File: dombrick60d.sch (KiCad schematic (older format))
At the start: 147 parts, among them J1 AVR-ISP-6, SW1 SW_Push, U1 ATmega32U2-AU, U2 PRTR5V0U2X, Y1 16MHz

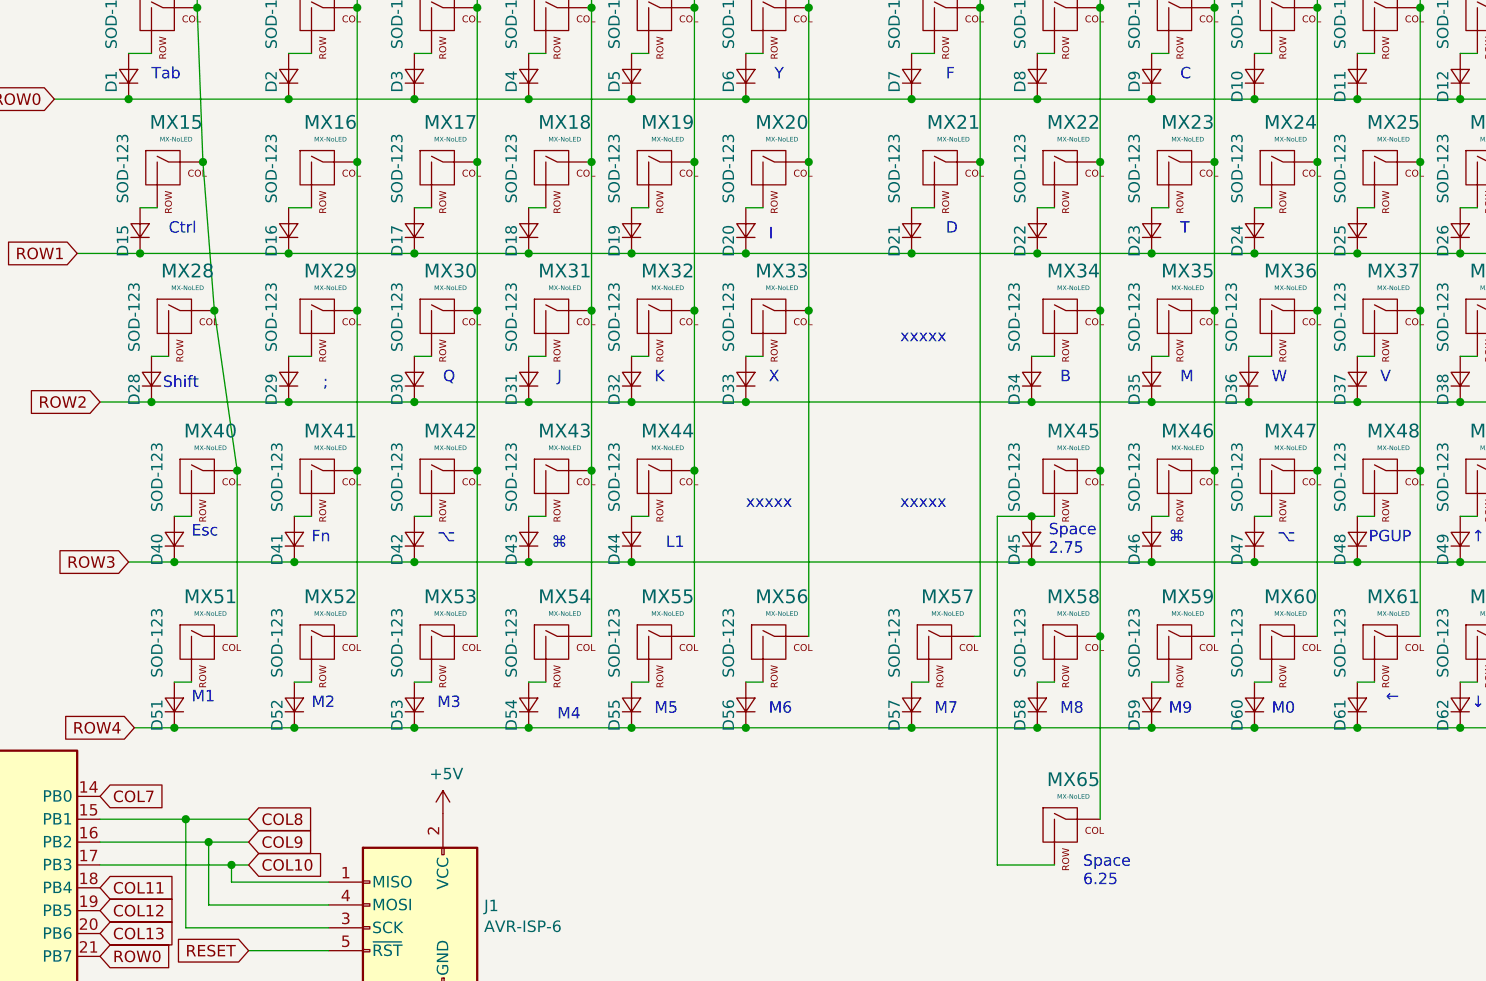
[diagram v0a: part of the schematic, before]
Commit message: sugee ganbatta
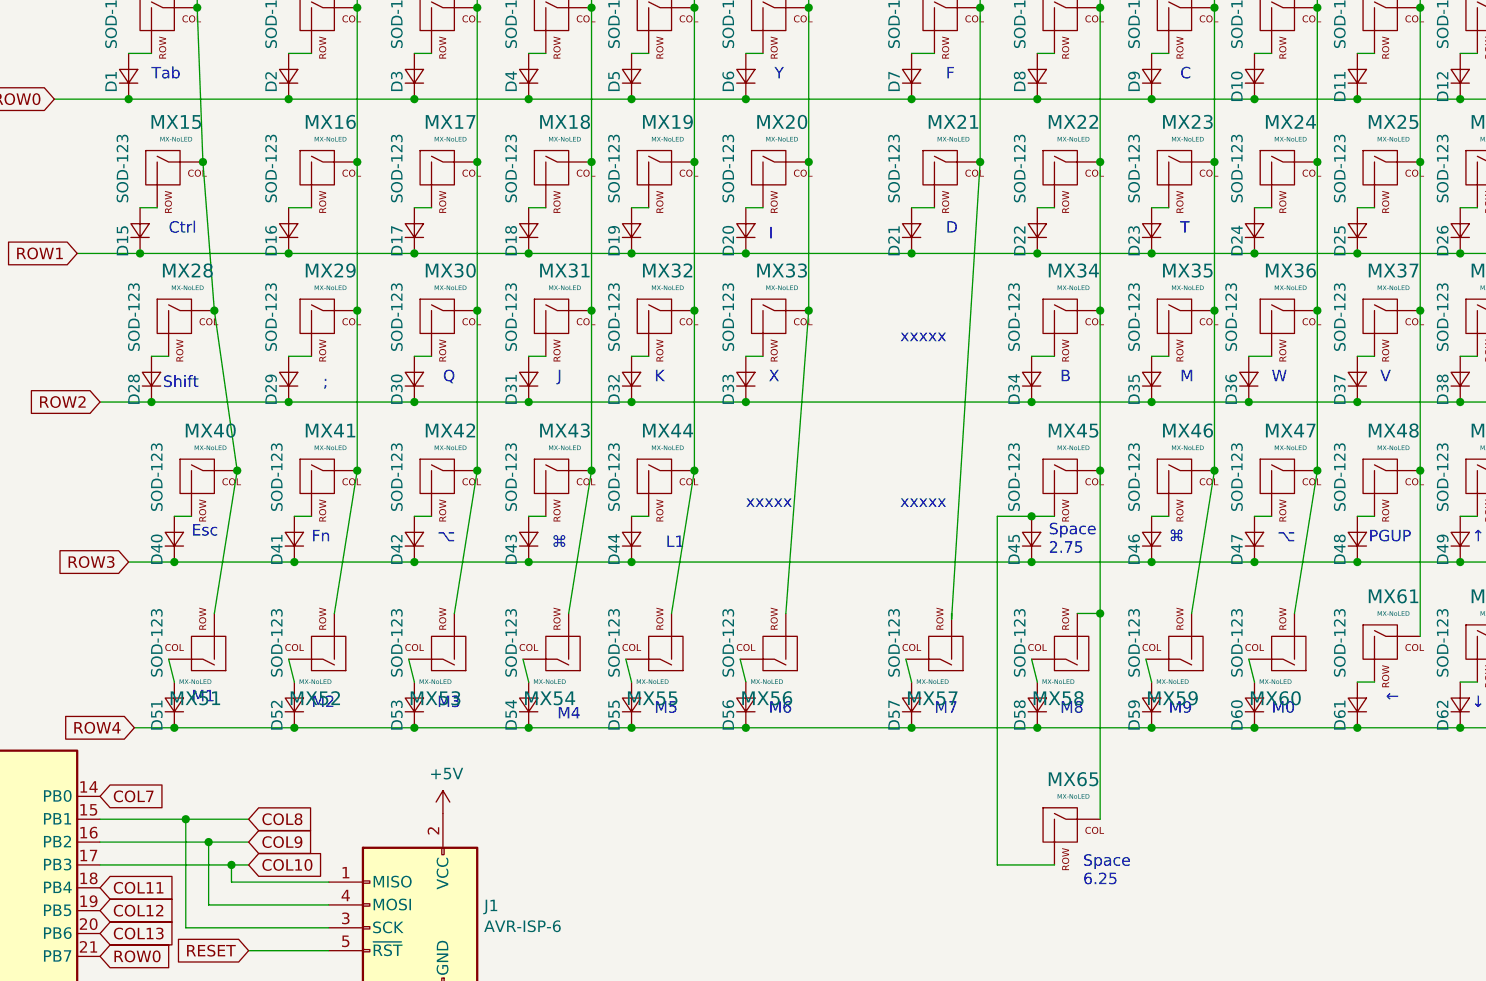
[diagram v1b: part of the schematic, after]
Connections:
- net COL0: now also MX51.2 (ROW); no longer MX51.1 (COL)
- net COL1: now also MX52.2 (ROW); no longer MX52.1 (COL)
- net COL2: now also MX53.2 (ROW); no longer MX53.1 (COL)
- net COL3: now also MX54.2 (ROW); no longer MX54.1 (COL)
- net COL4: now also MX55.2 (ROW); no longer MX55.1 (COL)
- net COL5: now also MX56.2 (ROW); no longer MX56.1 (COL)
- net COL6: now also MX57.2 (ROW); no longer MX57.1 (COL)
- net COL7: now also MX58.2 (ROW); no longer MX58.1 (COL)
- net COL8: now also MX59.2 (ROW); no longer MX59.1 (COL)
- net COL9: now also MX60.2 (ROW); no longer MX60.1 (COL)
- net at D55.2 (A): now also MX55.1 (COL); no longer MX55.2 (ROW)
- net at D59.2 (A): now also MX59.1 (COL); no longer MX59.2 (ROW)
- net at D60.2 (A): now also MX60.1 (COL); no longer MX60.2 (ROW)
- net at D51.2 (A): now also MX51.1 (COL); no longer MX51.2 (ROW)
- net at D52.2 (A): now also MX52.1 (COL); no longer MX52.2 (ROW)
- net at D53.2 (A): now also MX53.1 (COL); no longer MX53.2 (ROW)
- net at D54.2 (A): now also MX54.1 (COL); no longer MX54.2 (ROW)
- net at D56.2 (A): now also MX56.1 (COL); no longer MX56.2 (ROW)
- net at D57.2 (A): now also MX57.1 (COL); no longer MX57.2 (ROW)
- net at D58.2 (A): now also MX58.1 (COL); no longer MX58.2 (ROW)
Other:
- moved on the sheet: MX51, MX52, MX53, MX54, MX55, MX56, MX57, MX58, MX59, MX60
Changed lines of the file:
@@
 	9300 3600 9750 3600
 Wire Wire Line
-	8675 3200 8675 3925
+	8675 3200 8575 3825
 Wire Wire Line
 	8400 3400 8475 3400
@@
 Data
 89 50 4E 47 0D 0A 1A 0A 00 00 00 0D 49 48 44 52 00 00 01 AC 00 00 00 BB 08 02 00 00 00 B6 0E 3D
-6C 00 00 00 03 73 42 49 54 08 08 08 DB E1 4F E0 00 00 00 09 70 48 59 73 00 00 0B 12 00 00 0B 12
-01 D2 DD 7E FC 00 00 20 00 49 44 41 54 78 9C ED 9D 3F 7C 1A C9 15 C7 67 51 CA 58 0B E9 4F 80 7B
+6C 00 00 00 03 73 42 49 54 08 08 08 DB E1 4F E0 00 00 00 09 70 48 59 73 00 00 0A F0 00 00 0A F0
+01 42 AC 34 98 00 00 20 00 49 44 41 54 78 9C ED 9D 3F 7C 1A C9 15 C7 67 51 CA 58 0B E9 4F 80 7B
 F3 C7 9F B4 16 8B D2 0B AC 4B 1B 49 F8 EA 33 C8 57 5B 20 5F 9B 48 C8 A9 83 B0 9D 2E 9F 08 64 7F
 52 5A AC E4 94 39 81 7C 2E 73 06 E4 DE FC 71 CA 13 93 E2 99 F1 63 76 C1 48 62 97 85 7D DF 42 9F
@@
 F 3 "" H 5625 3950 60  0001 C CNN
 	1    6250 3975
-	1    0    0    -1
+	-1   0    0    1
 $EndComp
 $Comp
@@
 $EndComp
 Wire Wire Line
-	6125 4125 6200 4125
+	6125 4125 6100 4025
 Text Notes 6225 4275 0    50   ~ 0
 M5
@@
 $EndComp
 $Comp
-L MX_Alps_Hybrid:MX-NoLED MX?
-U 1 1 5E9D839C
-P 9425 3975
-AR Path="/5E22FDCD/5E9D839C" Ref="MX?"  Part="1"
-AR Path="/5E9D839C" Ref="MX61"  Part="1"
-F 0 "MX61" H 9458 4198 60  0000 C CNN
-F 1 "MX-NoLED" H 9458 4124 20  0000 C CNN
-F 2 "MX_Alps_Hybrid:MX-1U-NoLED" H 8800 3950 60  0001 C CNN
-F 3 "" H 8800 3950 60  0001 C CNN
-	1    9425 3975
-	1    0    0    -1
-$EndComp
-$Comp
 L Device:D_Small D?
 U 1 1 5E9D83A6
@@
 →
 Wire Wire Line
-	8850 4125 8925 4125
+	8850 4125 8825 4025
 $Comp
 L MX_Alps_Hybrid:MX-NoLED MX?
@@
 F 3 "" H 8350 3950 60  0001 C CNN
 	1    8975 3975
-	1    0    0    -1
+	-1   0    0    1
 $EndComp
 $Comp
@@
 F 3 "" H 7900 3950 60  0001 C CNN
 	1    8525 3975
-	1    0    0    -1
-$EndComp
-Wire Wire Line
-	8400 4125 8475 4125
+	-1   0    0    1
+$EndComp
+Wire Wire Line
+	8400 4125 8375 4025
 Text Notes 5800 4300 0    50   ~ 0
 M4
@@
 F 3 "" H 3625 3950 60  0001 C CNN
 	1    4250 3975
-	1    0    0    -1
+	-1   0    0    1
 $EndComp
 $Comp
@@
 $EndComp
 Wire Wire Line
-	4125 4125 4200 4125
+	4125 4125 4100 4025
 $Comp
 L MX_Alps_Hybrid:MX-NoLED MX?
@@
 F 3 "" H 4150 3950 60  0001 C CNN
 	1    4775 3975
-	1    0    0    -1
+	-1   0    0    1
 $EndComp
 $Comp
@@
 $EndComp
 Wire Wire Line
-	4650 4125 4725 4125
+	4650 4125 4625 4025
 $Comp
 L MX_Alps_Hybrid:MX-NoLED MX?
@@
 F 3 "" H 4675 3950 60  0001 C CNN
 	1    5300 3975
-	1    0    0    -1
+	-1   0    0    1
 $EndComp
 $Comp
@@
 $EndComp
 Wire Wire Line
-	5175 4125 5250 4125
+	5175 4125 5150 4025
 $Comp
 L MX_Alps_Hybrid:MX-NoLED MX?
@@
 F 3 "" H 5175 3950 60  0001 C CNN
 	1    5800 3975
-	1    0    0    -1
+	-1   0    0    1
 $EndComp
 $Comp
@@
 $EndComp
 Wire Wire Line
-	5675 4125 5750 4125
+	5675 4125 5650 4025
 Text Notes 4200 4225 0    50   ~ 0
 M1
@@
 F 3 "" H 6125 3950 60  0001 C CNN
 	1    6750 3975
-	1    0    0    -1
+	-1   0    0    1
 $EndComp
 $Comp
@@
 $EndComp
 Wire Wire Line
-	6625 4125 6700 4125
+	6625 4125 6600 4025
 Text Notes 6725 4275 0    50   ~ 0
 M6
@@
 F 3 "" H 6850 3950 60  0001 C CNN
 	1    7475 3975
-	1    0    0    -1
+	-1   0    0    1
 $EndComp
 $Comp
@@
 $EndComp
 Wire Wire Line
-	7350 4125 7425 4125
+	7350 4125 7325 4025
 Text Notes 7450 4275 0    50   ~ 0
 M7
@@
 F 3 "" H 7400 3950 60  0001 C CNN
 	1    8025 3975
-	1    0    0    -1
+	-1   0    0    1
 $EndComp
 $Comp
@@
 $EndComp
 Wire Wire Line
-	7900 4125 7975 4125
+	7900 4125 7875 4025
 Text Notes 8000 4275 0    50   ~ 0
 M8
@@
 	7900 4325 8400 4325
 Wire Wire Line
-	4400 3200 4400 3925
+	4400 3200 4300 3825
 Connection ~ 4400 3200
 Wire Wire Line
-	4925 3200 4925 3925
+	4925 3200 4825 3825
 Connection ~ 4925 3200
 Wire Wire Line
-	5450 3200 5450 3925
+	5450 3200 5350 3825
 Connection ~ 5450 3200
 Wire Wire Line
-	6900 3925 6900 2500
+	6800 3825 6900 2500
 Connection ~ 6900 2500
 Wire Wire Line
@@
 	11025 800  11025 1175
 Wire Wire Line
-	8175 3200 8175 3925
-Connection ~ 8175 3925
-Wire Wire Line
-	8175 3925 8175 4725
-Wire Wire Line
-	7650 3925 7625 3925
-Wire Wire Line
-	5950 3200 5950 3925
+	7525 3850 7525 3825
+Wire Wire Line
+	5950 3200 5850 3825
 Connection ~ 5950 3200
 Wire Wire Line
-	6400 3200 6400 3925
+	6400 3200 6300 3825
 Connection ~ 6400 3200
 Connection ~ 8175 3200
@@
 Connection ~ 7650 1850
 Wire Wire Line
-	7650 1850 7650 3925
+	7650 1850 7525 3850
 Text Notes 7300 2650 0    50   ~ 0
 xxxxx
 Wire Wire Line
-	9125 3200 9125 3925
+	9125 3200 9025 3825
 Connection ~ 9125 3200
 Wire Wire Line
@@
 Text GLabel 2100 4625 0    50   Input ~ 0
 RESET
+Wire Wire Line
+	8175 3200 8175 3825
+Wire Wire Line
+	8075 3825 8175 3825
+Connection ~ 8175 3825
+Wire Wire Line
+	8175 3825 8175 4725
+$Comp
+L MX_Alps_Hybrid:MX-NoLED MX?
+U 1 1 5E9D839C
+P 9425 3975
+AR Path="/5E22FDCD/5E9D839C" Ref="MX?"  Part="1"
+AR Path="/5E9D839C" Ref="MX61"  Part="1"
+F 0 "MX61" H 9458 4198 60  0000 C CNN
+F 1 "MX-NoLED" H 9458 4124 20  0000 C CNN
+F 2 "MX_Alps_Hybrid:MX-1U-NoLED" H 8800 3950 60  0001 C CNN
+F 3 "" H 8800 3950 60  0001 C CNN
+	1    9425 3975
+	1    0    0    -1
+$EndComp
 $EndSCHEMATC

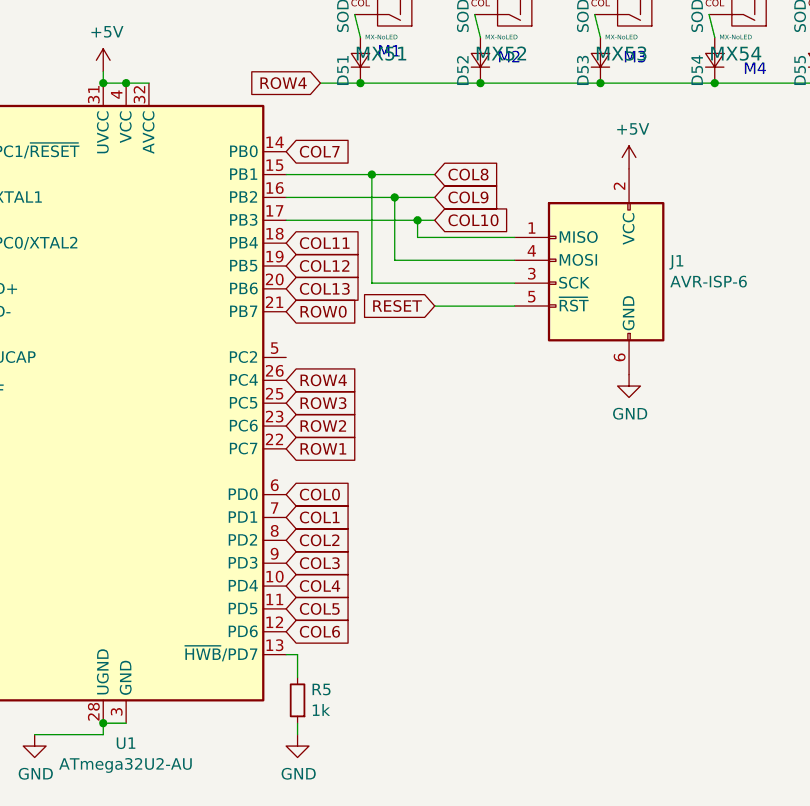
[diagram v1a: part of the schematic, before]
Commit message: sugoku ganbatta
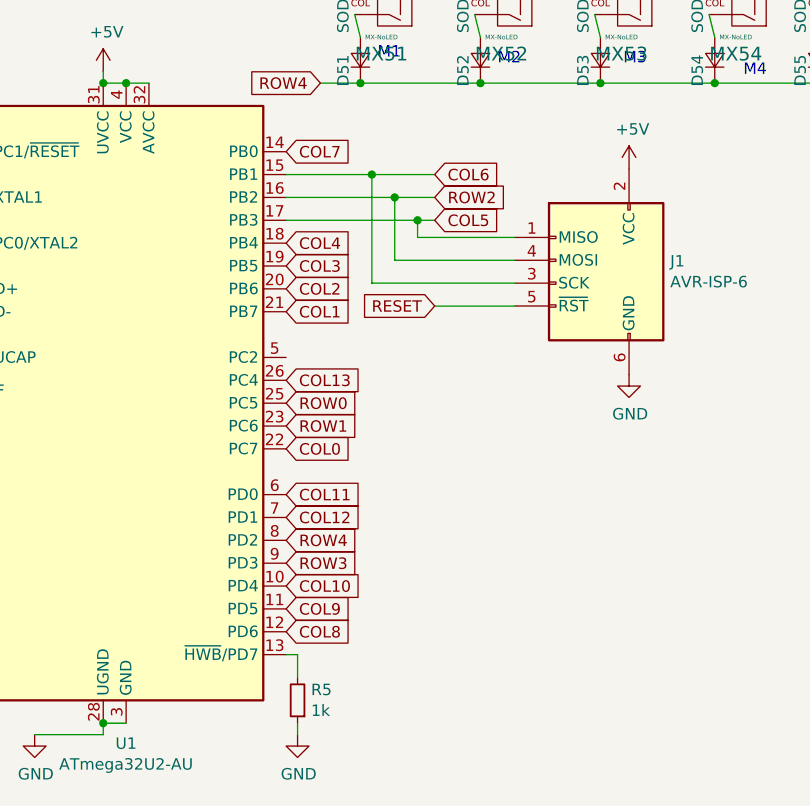
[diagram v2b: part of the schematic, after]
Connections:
- net COL0: now also U1.22 (PC7); no longer U1.6 (PD0)
- net COL1: now also U1.21 (PB7); no longer U1.7 (PD1)
- net COL10: now also U1.10 (PD4); no longer J1.1 (MISO), U1.17 (PB3)
- net COL11: now also U1.6 (PD0); no longer U1.18 (PB4)
- net COL12: now also U1.7 (PD1); no longer U1.19 (PB5)
- net COL13: now also U1.26 (PC4); no longer U1.20 (PB6)
- net COL2: now also U1.20 (PB6); no longer U1.8 (PD2)
- net COL3: now also U1.19 (PB5); no longer U1.9 (PD3)
- net COL4: now also U1.18 (PB4); no longer U1.10 (PD4)
- net COL5: now also J1.1 (MISO), U1.17 (PB3); no longer U1.11 (PD5)
- net COL6: now also J1.3 (SCK), U1.15 (PB1); no longer U1.12 (PD6)
- net COL8: now also U1.12 (PD6); no longer J1.3 (SCK), U1.15 (PB1)
- net COL9: now also U1.11 (PD5); no longer J1.4 (MOSI), U1.16 (PB2)
- net ROW0: now also U1.25 (PC5); no longer U1.21 (PB7)
- net ROW1: now also U1.23 (PC6); no longer U1.22 (PC7)
- net ROW2: now also J1.4 (MOSI), U1.16 (PB2); no longer U1.23 (PC6)
- net ROW3: now also U1.9 (PD3); no longer U1.25 (PC5)
- net ROW4: now also U1.8 (PD2); no longer U1.26 (PC4)
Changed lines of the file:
@@
 EESchema Schematic File Version 4
+LIBS:dombrick60d-cache
 EELAYER 30 0
 EELAYER END
@@
 	4450 5300 4800 5300
 Text GLabel 3800 6125 2    50   Input ~ 0
-COL0
+COL11
 Text GLabel 3800 6225 2    50   Input ~ 0
-COL1
-Text GLabel 3800 6325 2    50   Input ~ 0
-COL2
+COL12
 Text GLabel 3800 6425 2    50   Input ~ 0
-COL3
-Text GLabel 3800 6525 2    50   Input ~ 0
-COL4
-Text GLabel 3800 6625 2    50   Input ~ 0
-COL5
+ROW3
 Text GLabel 3800 6725 2    50   Input ~ 0
-COL6
+COL8
 Text GLabel 3800 4625 2    50   Input ~ 0
 COL7
 Text GLabel 4450 4725 2    50   Input ~ 0
-COL8
+COL6
 Text GLabel 4450 4825 2    50   Input ~ 0
-COL9
+ROW2
 Text GLabel 4450 4925 2    50   Input ~ 0
-COL10
+COL5
 Wire Wire Line
 	4450 4725 4175 4725
@@
 Connection ~ 4375 4925
 Text GLabel 3800 5025 2    50   Input ~ 0
-COL11
+COL4
 Text GLabel 3800 5125 2    50   Input ~ 0
-COL12
+COL3
 Text GLabel 3800 5225 2    50   Input ~ 0
-COL13
-Text GLabel 3800 5325 2    50   Input ~ 0
-ROW0
-Text GLabel 3800 5925 2    50   Input ~ 0
-ROW1
+COL2
 Text GLabel 3800 5825 2    50   Input ~ 0
-ROW2
+ROW1
 Text GLabel 3800 5725 2    50   Input ~ 0
-ROW3
+ROW0
 Text GLabel 3800 5625 2    50   Input ~ 0
-ROW4
+COL13
 Text GLabel 2100 4625 0    50   Input ~ 0
 RESET
@@
 	1    0    0    -1
 $EndComp
+Text GLabel 3800 6325 2    50   Input ~ 0
+ROW4
+Text GLabel 3800 5325 2    50   Input ~ 0
+COL1
+Text GLabel 3800 5925 2    50   Input ~ 0
+COL0
+Text GLabel 3800 6525 2    50   Input ~ 0
+COL10
+Text GLabel 3800 6625 2    50   Input ~ 0
+COL9
 $EndSCHEMATC

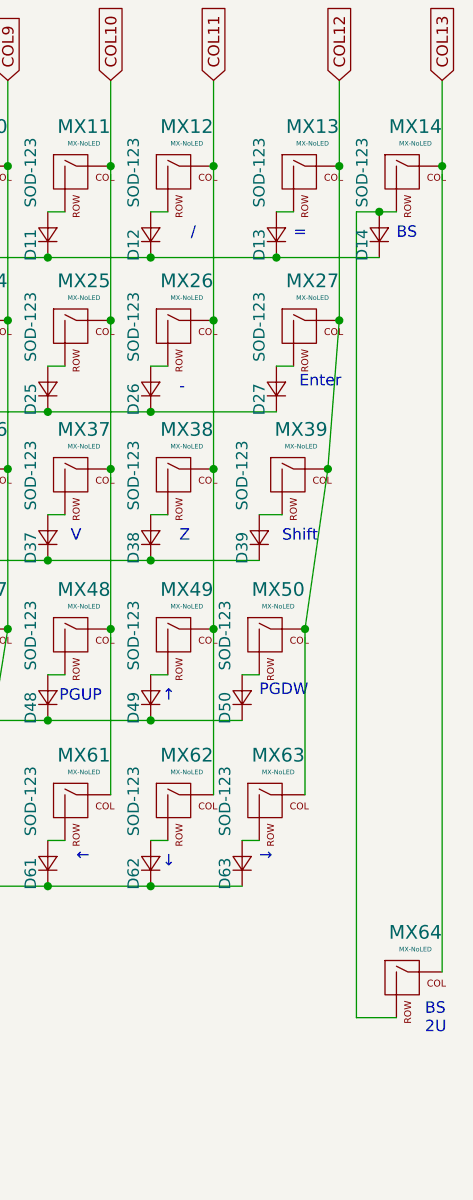
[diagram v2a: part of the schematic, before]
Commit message: 2020-01-19 all ok lets production start
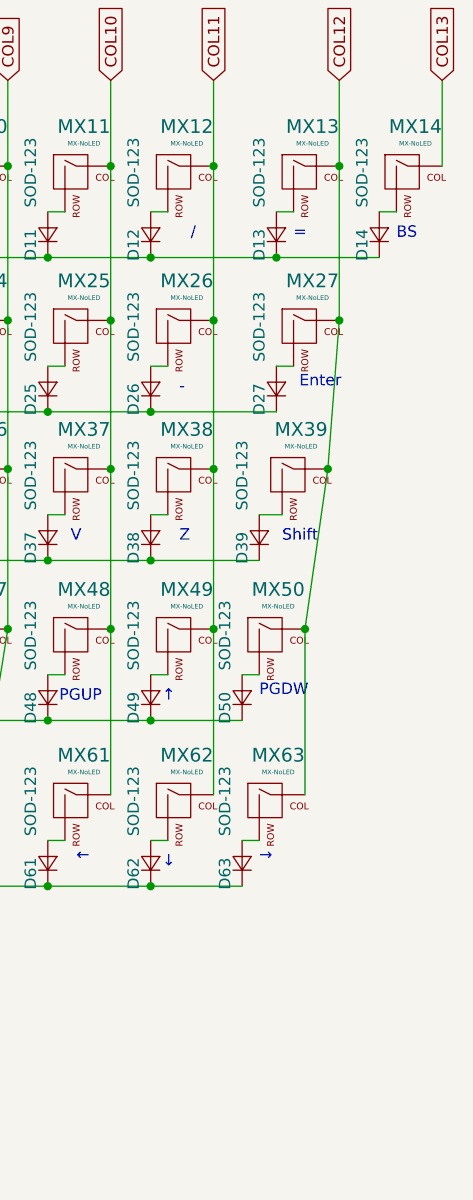
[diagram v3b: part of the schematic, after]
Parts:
- removed MX64: MX-NoLED, MX_Alps_Hybrid:MX-2U-NoLED, symbol MX_Alps_Hybrid:MX-NoLED
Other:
- note removed: "BS\n2U"
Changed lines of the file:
@@
 Text Notes 8100 5025 0    50   ~ 0
 Space\n6.25
-$Comp
-L MX_Alps_Hybrid:MX-NoLED MX?
-U 1 1 5F113CF0
-P 10875 4750
-AR Path="/5E22FDCD/5F113CF0" Ref="MX?"  Part="1"
-AR Path="/5F113CF0" Ref="MX64"  Part="1"
-F 0 "MX64" H 10908 4973 60  0000 C CNN
-F 1 "MX-NoLED" H 10908 4899 20  0000 C CNN
-F 2 "MX_Alps_Hybrid:MX-2U-NoLED" H 10250 4725 60  0001 C CNN
-F 3 "" H 10250 4725 60  0001 C CNN
-	1    10875 4750
-	1    0    0    -1
-$EndComp
-Wire Wire Line
-	11025 1175 11025 4700
-Connection ~ 11025 1175
-Wire Wire Line
-	10825 4900 10650 4900
-Wire Wire Line
-	10650 4900 10650 1375
-Wire Wire Line
-	10650 1375 10750 1375
-Connection ~ 10750 1375
-Text Notes 10950 4975 0    50   ~ 0
-BS\n2U
 Text GLabel 4225 800  1    50   Input ~ 0
 COL0
